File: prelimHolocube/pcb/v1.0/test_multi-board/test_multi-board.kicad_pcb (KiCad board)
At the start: 2 copper layers, 123.6 x 111.8 mm, 63 parts, among them J1 Breakout_1, J2 Breakout_2, J3 Breakout_3, J4 Breakout_4, J5 Breakout_5, J6 Breakout_6, J7 Breakout_7, J8 Breakout_8

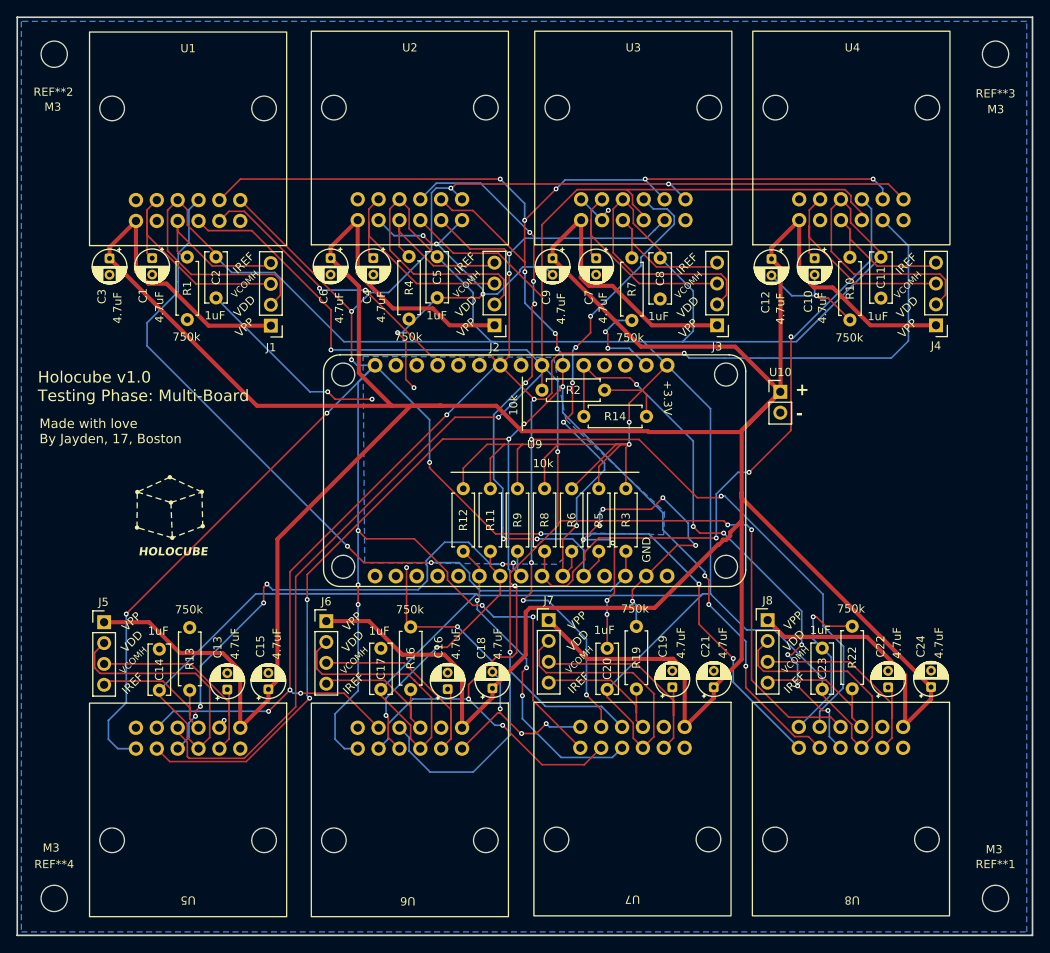
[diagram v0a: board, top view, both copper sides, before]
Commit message: order multiboard and update full board
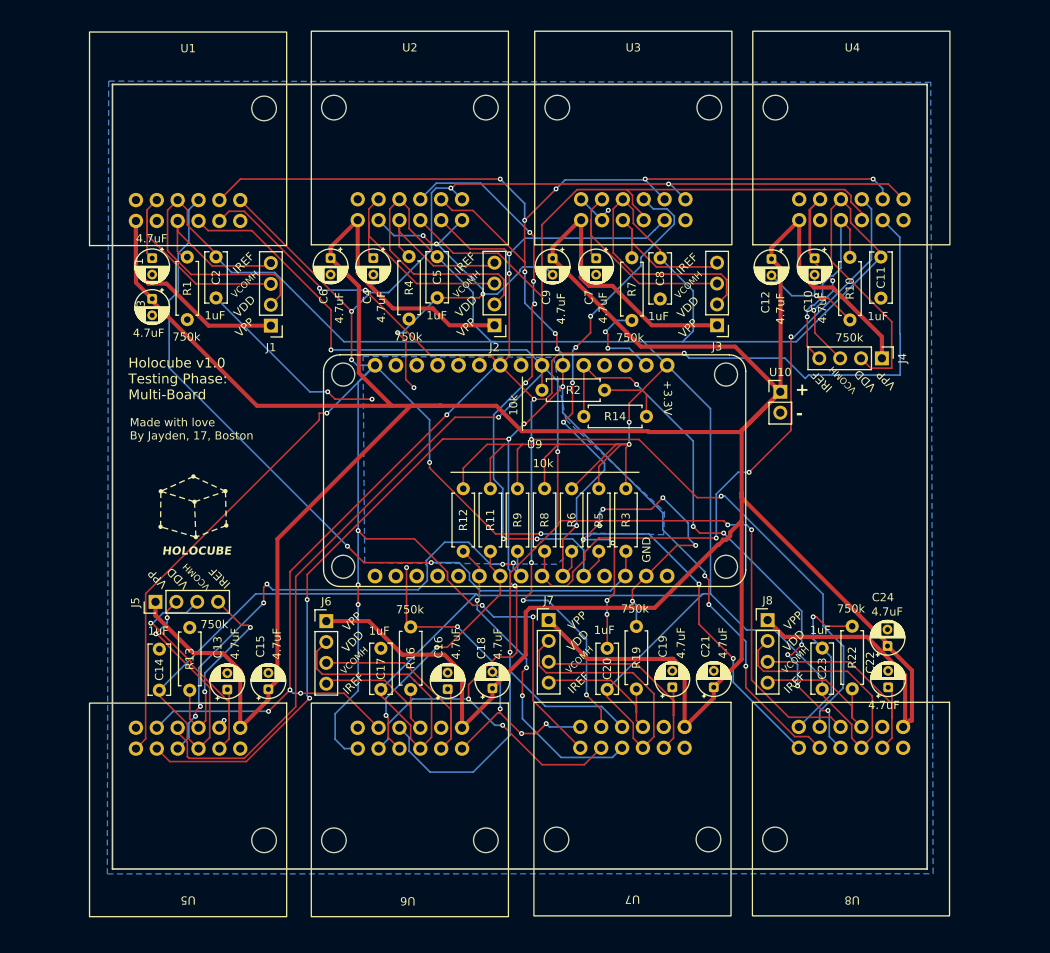
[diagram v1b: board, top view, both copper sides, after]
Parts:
- removed REF**1, REF**2, REF**3, REF**4: MountingHole_3.2mm_M3, MountingHole:MountingHole_3.2mm_M3
- moved J4 7.72 mm to (198.8, 81.8), turned to -90 degrees
- moved C24 7.29 mm to (199.4, 116.8)
- moved C3 7.16 mm to (109.9, 74.6)
- moved J5 6.73 mm to (110.3, 111.5), turned to 90 degrees
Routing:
- net VPP_1: track 580.8 -> 568.8 mm
- net IREF_5: track 17.9 -> 25.2 mm, vias 0 -> 2
- net IREF_4: track 18.1 -> 24.4 mm, vias 0 -> 1
- net VCOMH_4: track 27.2 -> 31.3 mm, vias 0 -> 2
- net SI: track 348.4 -> 344.9 mm, vias 15 -> 14
- net VCOMH_5: track 26.4 -> 29.7 mm, vias 0 -> 1
- net SCL: track 349.6 -> 352.6 mm
- net CS_1: track 95.2 -> 93.0 mm
- net VDD_1: track 636.2 -> 634.6 mm, vias 2 -> 4
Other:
- board size 123.6 x 111.8 mm -> 99.2 x 95.5 mm
- board text removed: "M3"
